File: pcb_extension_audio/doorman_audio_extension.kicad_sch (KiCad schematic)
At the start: 34 parts, among them J1 Audio Out, J4 Extension Board Connector, J5 Audio In, U1 ES8388

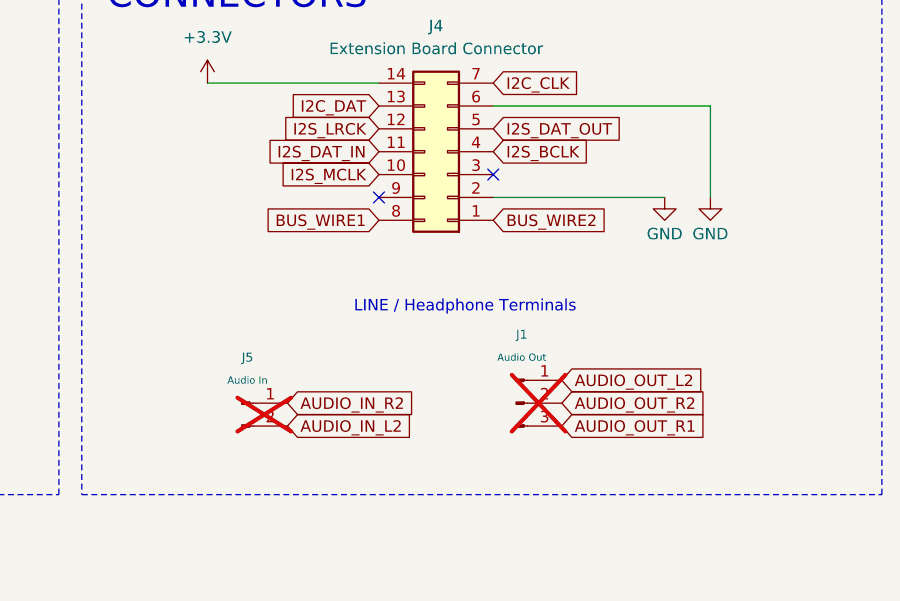
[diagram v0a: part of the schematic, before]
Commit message: WIP
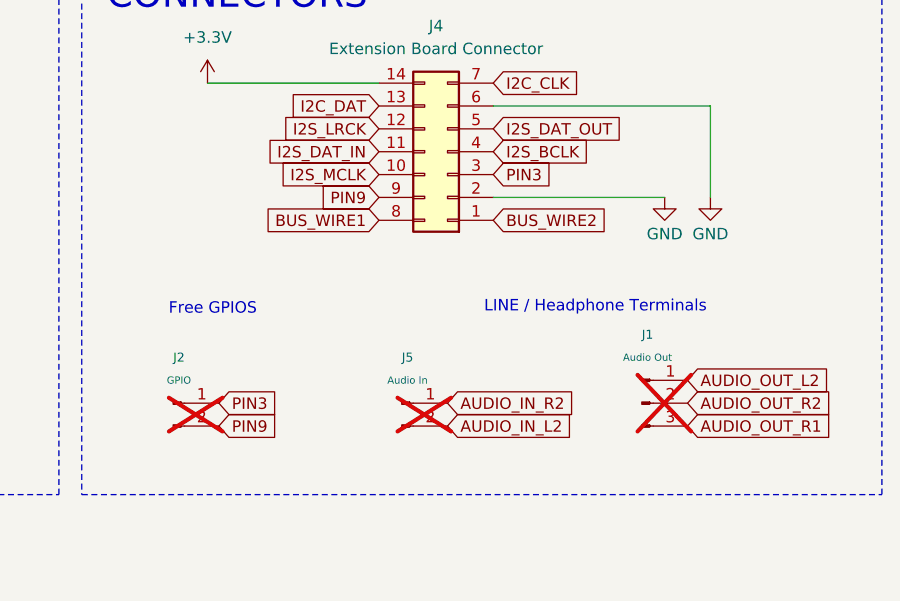
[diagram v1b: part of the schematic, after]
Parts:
- added J2: GPIO, Connector_PinHeader_2.54mm:PinHeader_1x02_P2.54mm_Vertical, symbol Connector:Conn_01x02_Pin
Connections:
- net PIN3: now reaches J4.3 (Pin_3)
- net PIN3: now also J2.1 (Pin_1)
- net PIN9: now reaches J4.9 (Pin_9)
- net PIN9: now also J2.2 (Pin_2)
- no-connect marks 2 -> 0
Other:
- note added: "Free GPIOS"
- moved on the sheet: J1, J5
